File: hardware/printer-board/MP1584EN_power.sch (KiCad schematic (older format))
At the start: 8 parts, among them U14 AMS1117-3.3

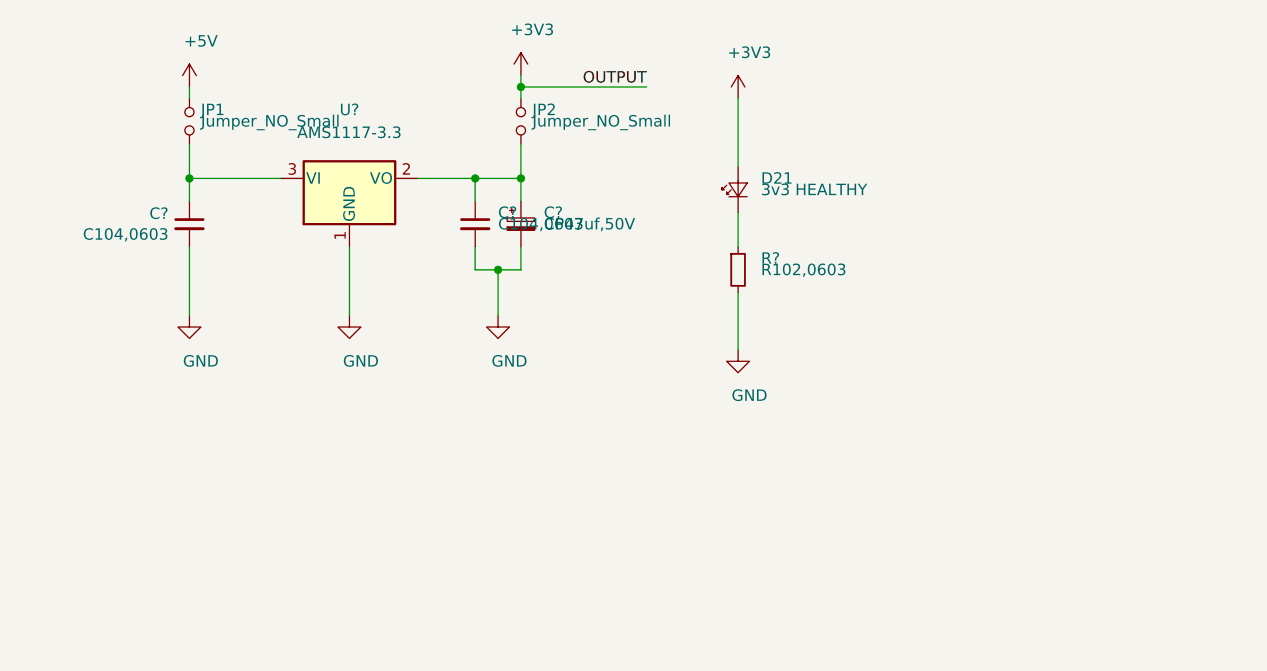
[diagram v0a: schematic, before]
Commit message: update,
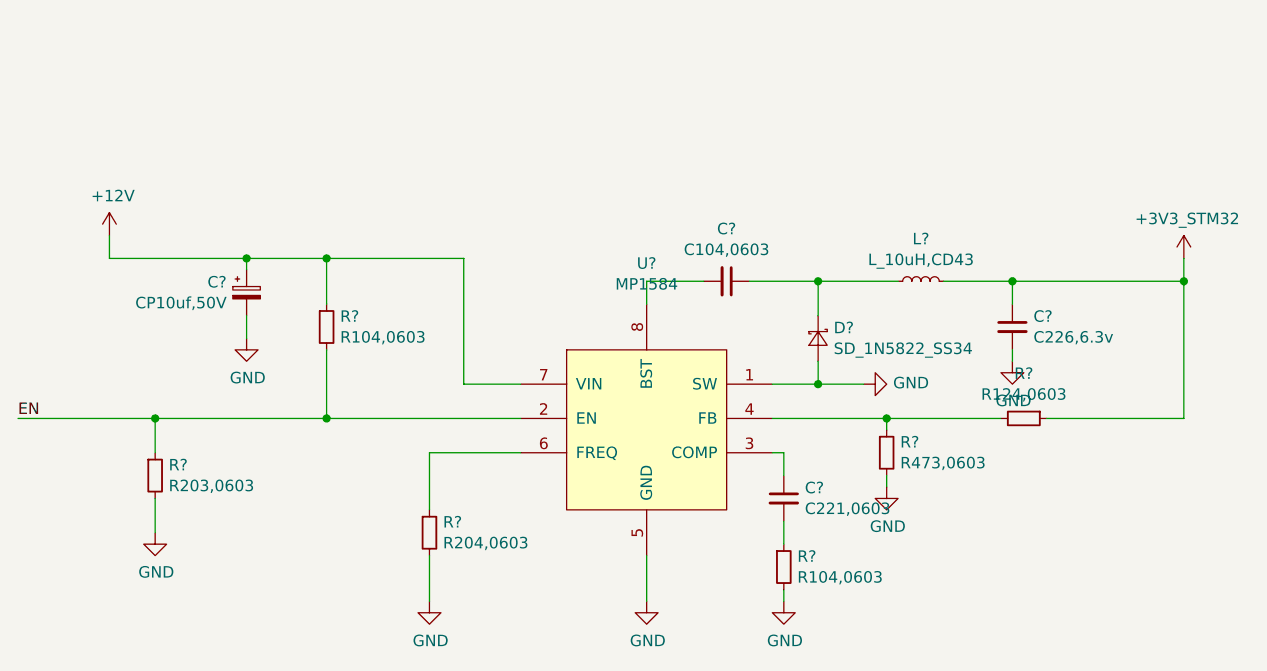
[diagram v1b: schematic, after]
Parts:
- removed C37, C38: C104,0603, Capacitor_SMD:C_0603_1608Metric_Pad1.05x0.95mm_HandSolder, symbol taobao-c:C104,0603
- removed C39: CP47uf,50V, w_smd_cap:c_elec_6.3x7.7, symbol taobao-cp:CP47uf,50V
- removed D21: 3v3 HEALTHY, LED_SMD:LED_0603_1608Metric_Pad1.05x0.95mm_HandSolder, symbol taobao-led:LED_GREEN,0603
- removed JP1, JP2: Jumper_NO_Small, Jumper:SolderJumper-2_P1.3mm_Bridged2Bar_RoundedPad1.0x1.5mm, symbol Device:Jumper_NO_Small
- removed R65: R102,0603, Resistor_SMD:R_0603_1608Metric_Pad1.05x0.95mm_HandSolder, symbol taobao-r:R102,0603
- removed U14: AMS1117-3.3, Package_TO_SOT_SMD:SOT-223-3_TabPin2, symbol Regulator_Linear:AMS1117-3.3
- added C?: CP10uf,50V, Capacitor_SMD:CP_Elec_5x5.3, symbol taobao-cp:CP10uf,50V
- added C?: C104,0603, Capacitor_SMD:C_0603_1608Metric_Pad1.05x0.95mm_HandSolder, symbol taobao-c:C104,0603
- added C?: C226,6.3v, symbol taobao-c:C226,6.3v
- added C?: C221,0603, Capacitor_SMD:C_0603_1608Metric_Pad1.05x0.95mm_HandSolder, symbol taobao-c:C221,0603
- added D?: SD_1N5822_SS34, symbol taobao-sd:SD_1N5822_SS34
- added L?: L_10uH,CD43, w_smd_inductors:inductor_smd_4.8x2.8mm, symbol taobao-l:L_10uH,CD43
- added R? (x2): R104,0603, Resistor_SMD:R_0603_1608Metric_Pad1.05x0.95mm_HandSolder, symbol taobao-r:R104,0603
- added R?: R204,0603, Resistor_SMD:R_0603_1608Metric_Pad1.05x0.95mm_HandSolder, symbol taobao-r:R204,0603
- added R?: R203,0603, Resistor_SMD:R_0603_1608Metric_Pad1.05x0.95mm_HandSolder, symbol taobao-r:R203,0603
- added R?: R473,0603, Resistor_SMD:R_0603_1608Metric_Pad1.05x0.95mm_HandSolder, symbol taobao-r:R473,0603
- added R?: R124,0603, Resistor_SMD:R_0603_1608Metric_Pad1.05x0.95mm_HandSolder, symbol taobao-r:R124,0603
- added U?: MP1584, symbol taobao-components:MP1584
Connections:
- net GND: now also C?.2, C?.2, D?.2 (A), R?.2, R?.2, R?.2, R?.2, U?.1 (SW), U?.5 (GND)
- new net: C?.1, U?.3 (COMP)
- new net: R?.1, R?.2, U?.4 (FB)
- new net: R?.1, U?.6 (FREQ)
- new net: C?.2, U?.8 (BST)
- new net: C?.1, D?.1 (K), L?.1
- new net: C?.2, R?.1
- new net +12V: C?.1, R?.1, U?.7 (VIN)
- new net +3V3_STM32: C?.1, L?.2, R?.1
- new net EN: R?.1, R?.2, U?.2 (EN)
